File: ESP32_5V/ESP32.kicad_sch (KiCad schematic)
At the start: 3 parts, among them J2 Conn_01x15, J3 Conn_01x15

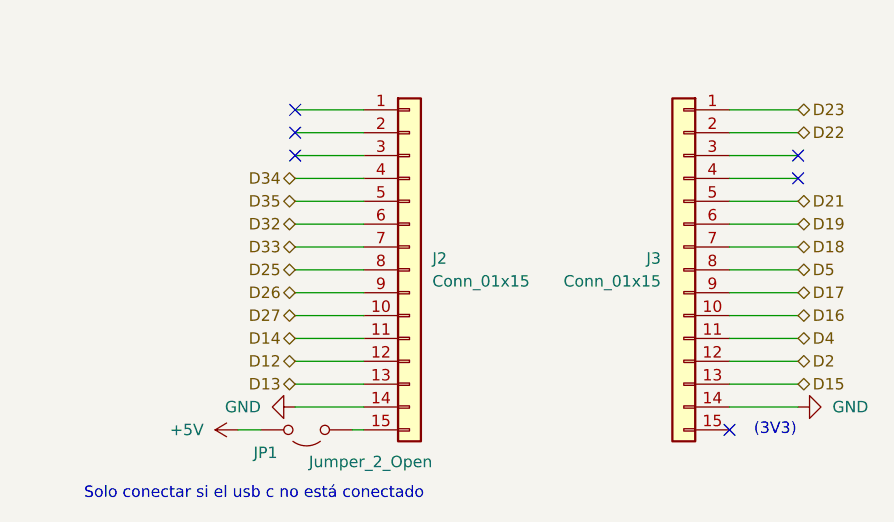
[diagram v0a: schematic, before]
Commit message: update
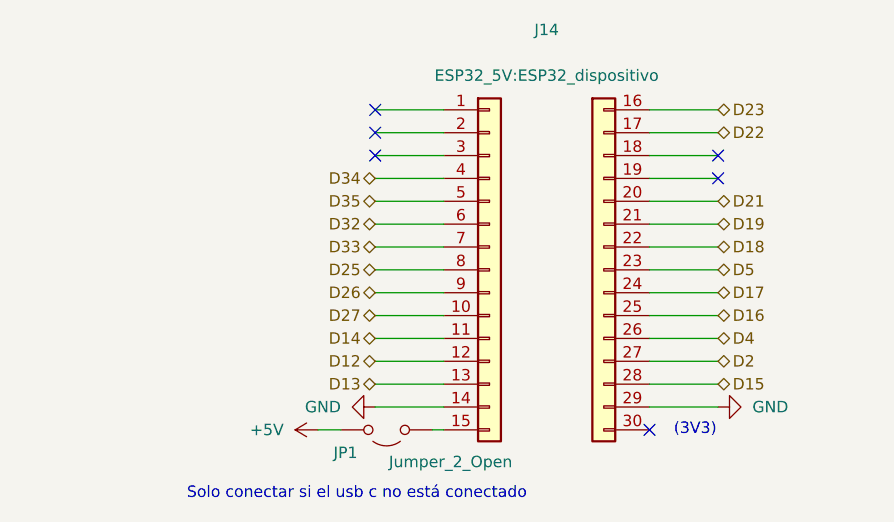
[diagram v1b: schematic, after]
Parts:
- removed J2, J3: Conn_01x15, Connector_PinSocket_2.54mm:PinSocket_1x15_P2.54mm_Vertical, symbol Connector_Generic:Conn_01x15
- added J14: ~, ESP32_5V:ESP32_dispositivo, symbol ESP32_5v_library:esp32_board_pins
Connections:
- net D12: now also J14.12
- net D13: now also J14.13
- net D14: now also J14.11
- net D15: now also J14.28
- net D16: now also J14.25
- net D17: now also J14.24
- net D18: now also J14.22
- net D19: now also J14.21
- net D2: now also J14.27
- net D21: now also J14.20
- net D22: now also J14.17
- net D23: now also J14.16
- net D25: now also J14.8
- net D26: now also J14.9
- net D27: now also J14.10
- net D32: now also J14.6
- net D33: now also J14.7
- net D34: now also J14.4
- net D35: now also J14.5
- net D4: now also J14.26
- net D5: now also J14.23
- net GND: now also J14.14, J14.29
- net at JP1.1 (A): now also J14.15
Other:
- moved on the sheet: JP1
